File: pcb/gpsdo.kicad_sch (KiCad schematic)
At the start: 10 parts, among them U1 CD74HC390, U2 ATtiny3217-M, U3 MC74HC4046, U4 OCS52A

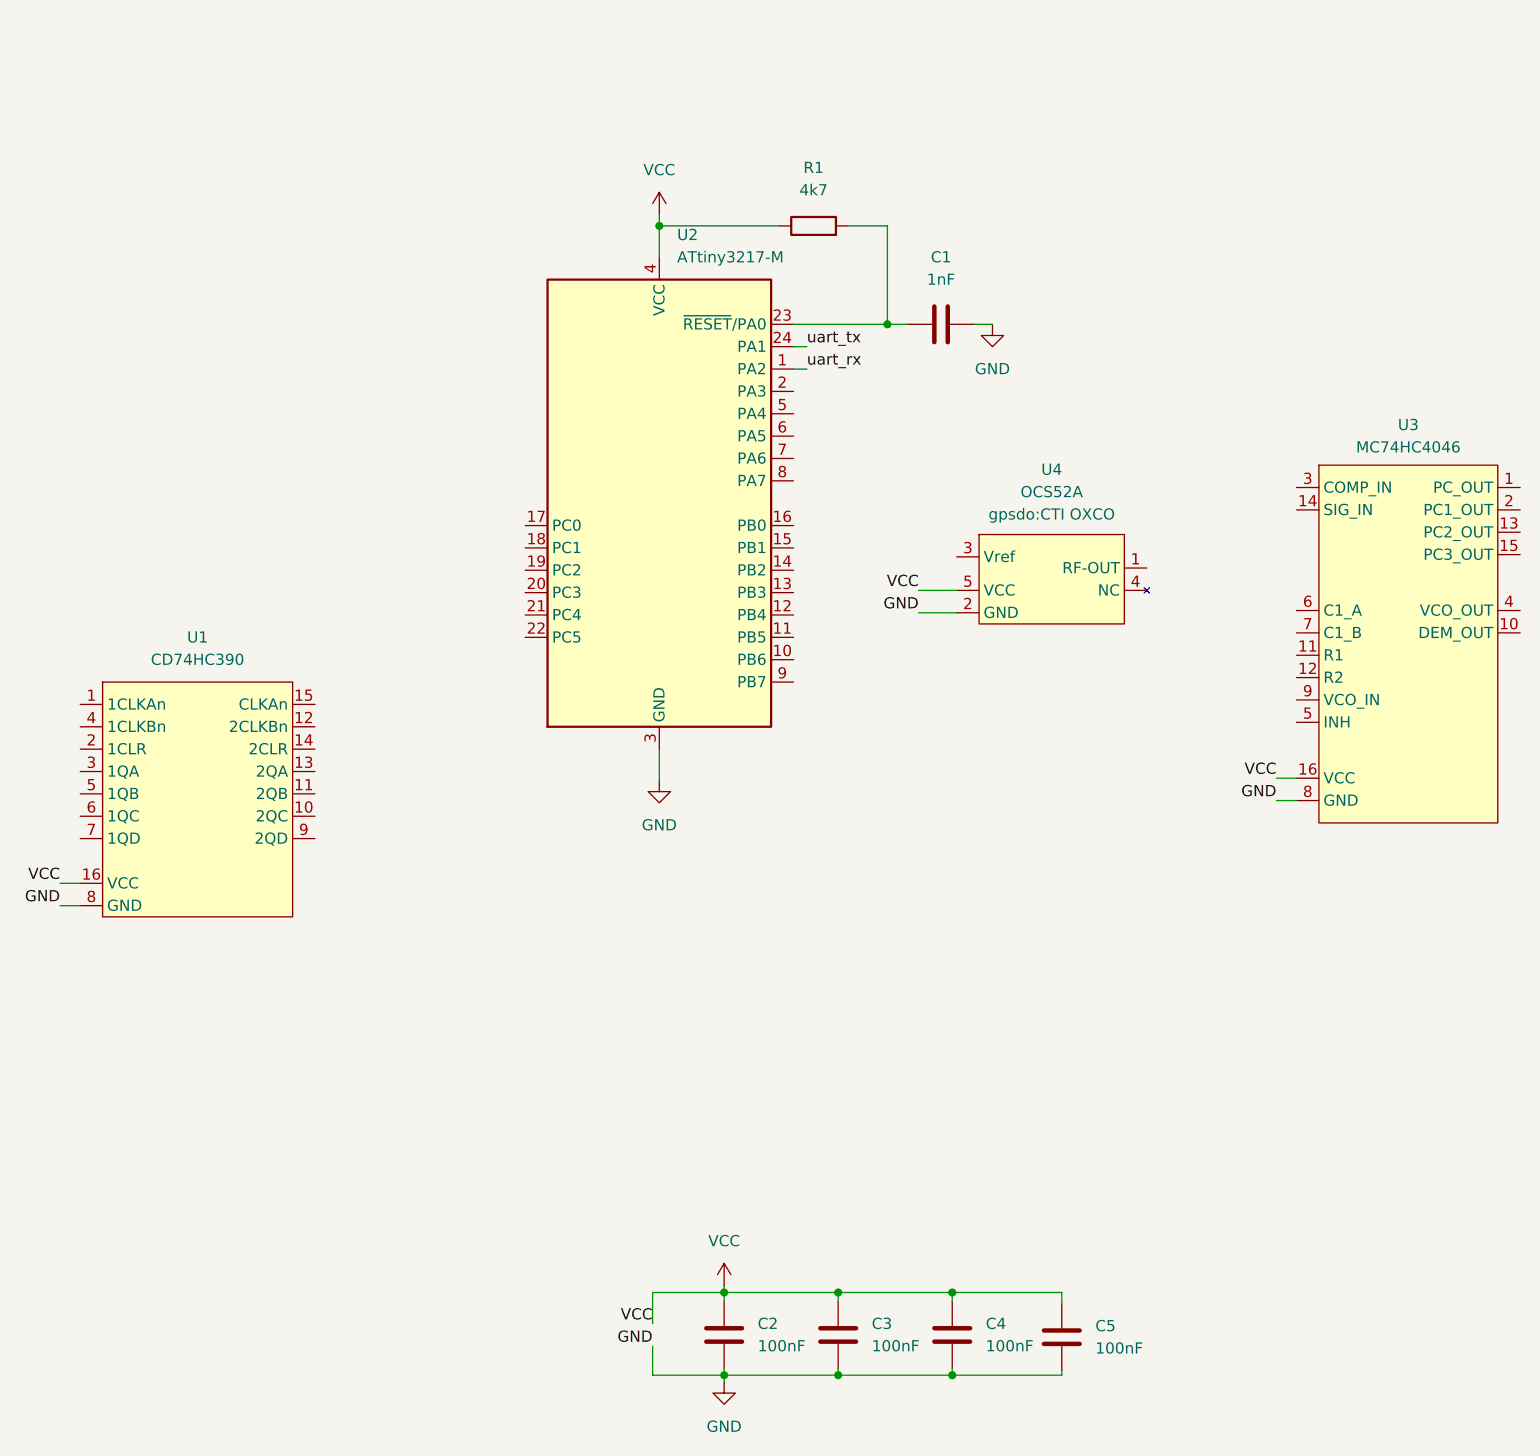
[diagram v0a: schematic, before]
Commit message: started layout
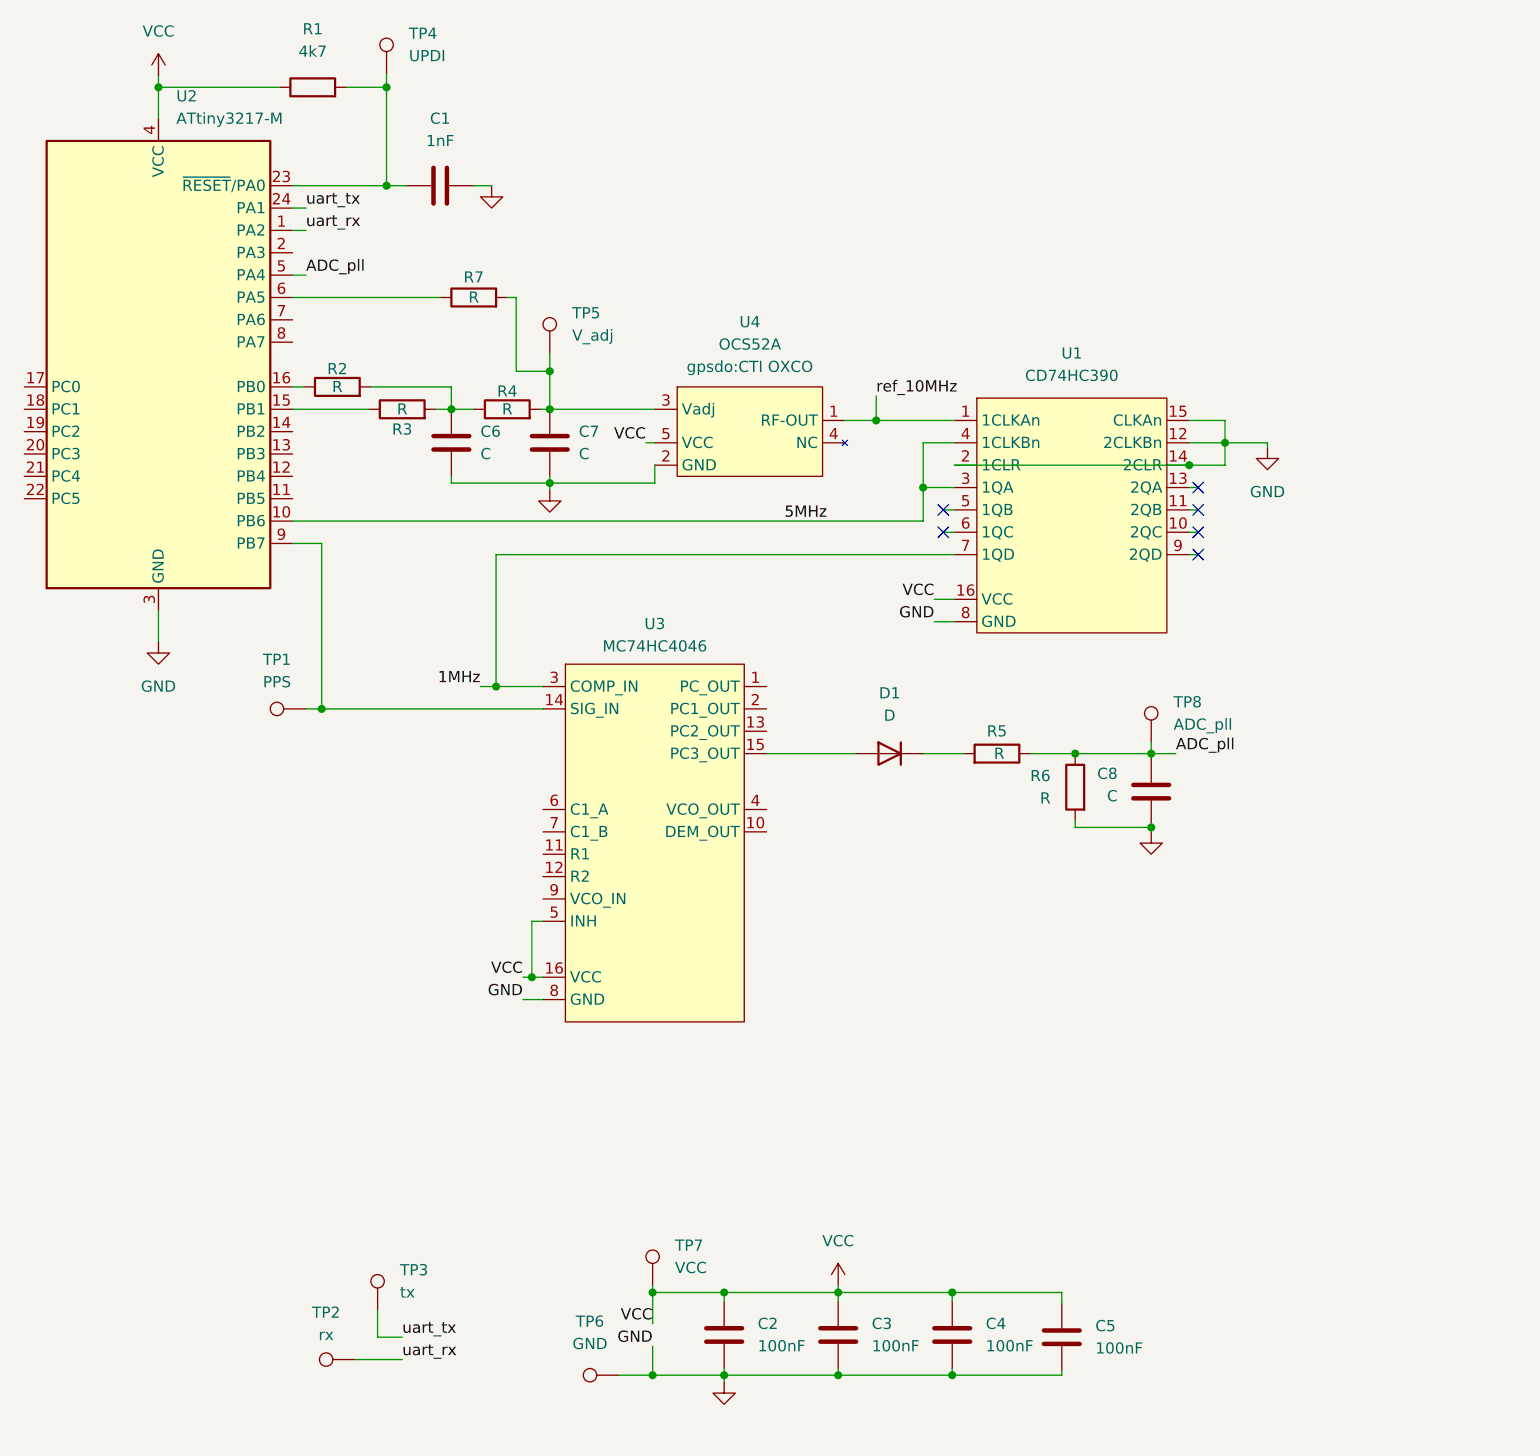
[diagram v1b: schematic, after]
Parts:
- added C6, C7, C8: C, Capacitor_SMD:C_0805_2012Metric_Pad1.18x1.45mm_HandSolder, symbol Device:C
- added D1: D, Diode_THT:D_DO-35_SOD27_P2.54mm_Vertical_KathodeUp, symbol Device:D
- added R2, R3, R4, R5, R6, R7: R, Resistor_SMD:R_0805_2012Metric_Pad1.20x1.40mm_HandSolder, symbol Device:R
- added TP1: PPS, TestPoint:TestPoint_Loop_D1.80mm_Drill1.0mm_Beaded, symbol Connector:TestPoint
- added TP2: rx, TestPoint:TestPoint_Loop_D1.80mm_Drill1.0mm_Beaded, symbol Connector:TestPoint
- added TP3: tx, TestPoint:TestPoint_Loop_D1.80mm_Drill1.0mm_Beaded, symbol Connector:TestPoint
- added TP4: UPDI, TestPoint:TestPoint_Loop_D1.80mm_Drill1.0mm_Beaded, symbol Connector:TestPoint
- added TP5: V_adj, TestPoint:TestPoint_Pad_2.0x2.0mm, symbol Connector:TestPoint
- added TP6: GND, TestPoint:TestPoint_Loop_D1.80mm_Drill1.0mm_Beaded, symbol Connector:TestPoint
- added TP7: VCC, TestPoint:TestPoint_Loop_D1.80mm_Drill1.0mm_Beaded, symbol Connector:TestPoint
- added TP8: ADC_pll, TestPoint:TestPoint_Pad_2.0x2.0mm, symbol Connector:TestPoint
- C2, C3: footprint Resistor_SMD:R_0805_2012Metric_Pad1.20x1.40mm_HandSolder -> Capacitor_SMD:C_0805_2012Metric_Pad1.18x1.45mm_HandSolder
- R1: footprint Capacitor_SMD:C_0805_2012Metric_Pad1.18x1.45mm_HandSolder -> Resistor_SMD:R_0805_2012Metric_Pad1.20x1.40mm_HandSolder
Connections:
- net GND: now also U1.12 (2CLKBn), U1.14 (2CLR), U1.15 (CLKAn), U1.2 (1CLR), C6.2, C7.2, C8.2, R6.2, TP6.1
- net VCC: now also U3.5 (INH), TP7.1
- net uart_rx: now also TP2.1
- net uart_tx: now also TP3.1
- net at U3.14 (SIG_IN): now also U2.9 (PB7), TP1.1
- net at U3.15 (PC3_OUT): now also D1.2 (A)
- net 1MHz: now reaches U3.3 (COMP_IN)
- net 1MHz: now also U1.7 (1QD)
- net at C1.1, R1.2, U2.23 (~{RESET}/PA0): now also TP4.1
- net ref_10MHz: now reaches U1.1 (1CLKAn)
- net ref_10MHz: now also U4.1 (RF-OUT)
- net 5MHz: now reaches U1.3 (1QA)
- net 5MHz: now also U1.4 (1CLKBn), U2.10 (PB6)
- net at U2.15 (PB1): now also R3.1
- net at U2.16 (PB0): now also R2.1
- net ADC_pll: now reaches U2.5 (PA4)
- net ADC_pll: now also C8.1, R5.1, R6.1, TP8.1
- net at U2.6 (PA5): now also R7.1
- net at U4.3 (Vadj): now also C7.1, R4.2, R7.2, TP5.1
- new net: C6.1, R2.2, R3.2, R4.1
- new net: D1.1 (K), R5.2
- no-connect marks 0 -> 6
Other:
- moved on the sheet: C1, R1, U1, U2, U3, U4
